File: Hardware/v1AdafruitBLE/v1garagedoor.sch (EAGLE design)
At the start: 28 parts, among them IC1 78V, Q1 2N3904, U1 ATMEGA328P_PDIP, X1 16mhz

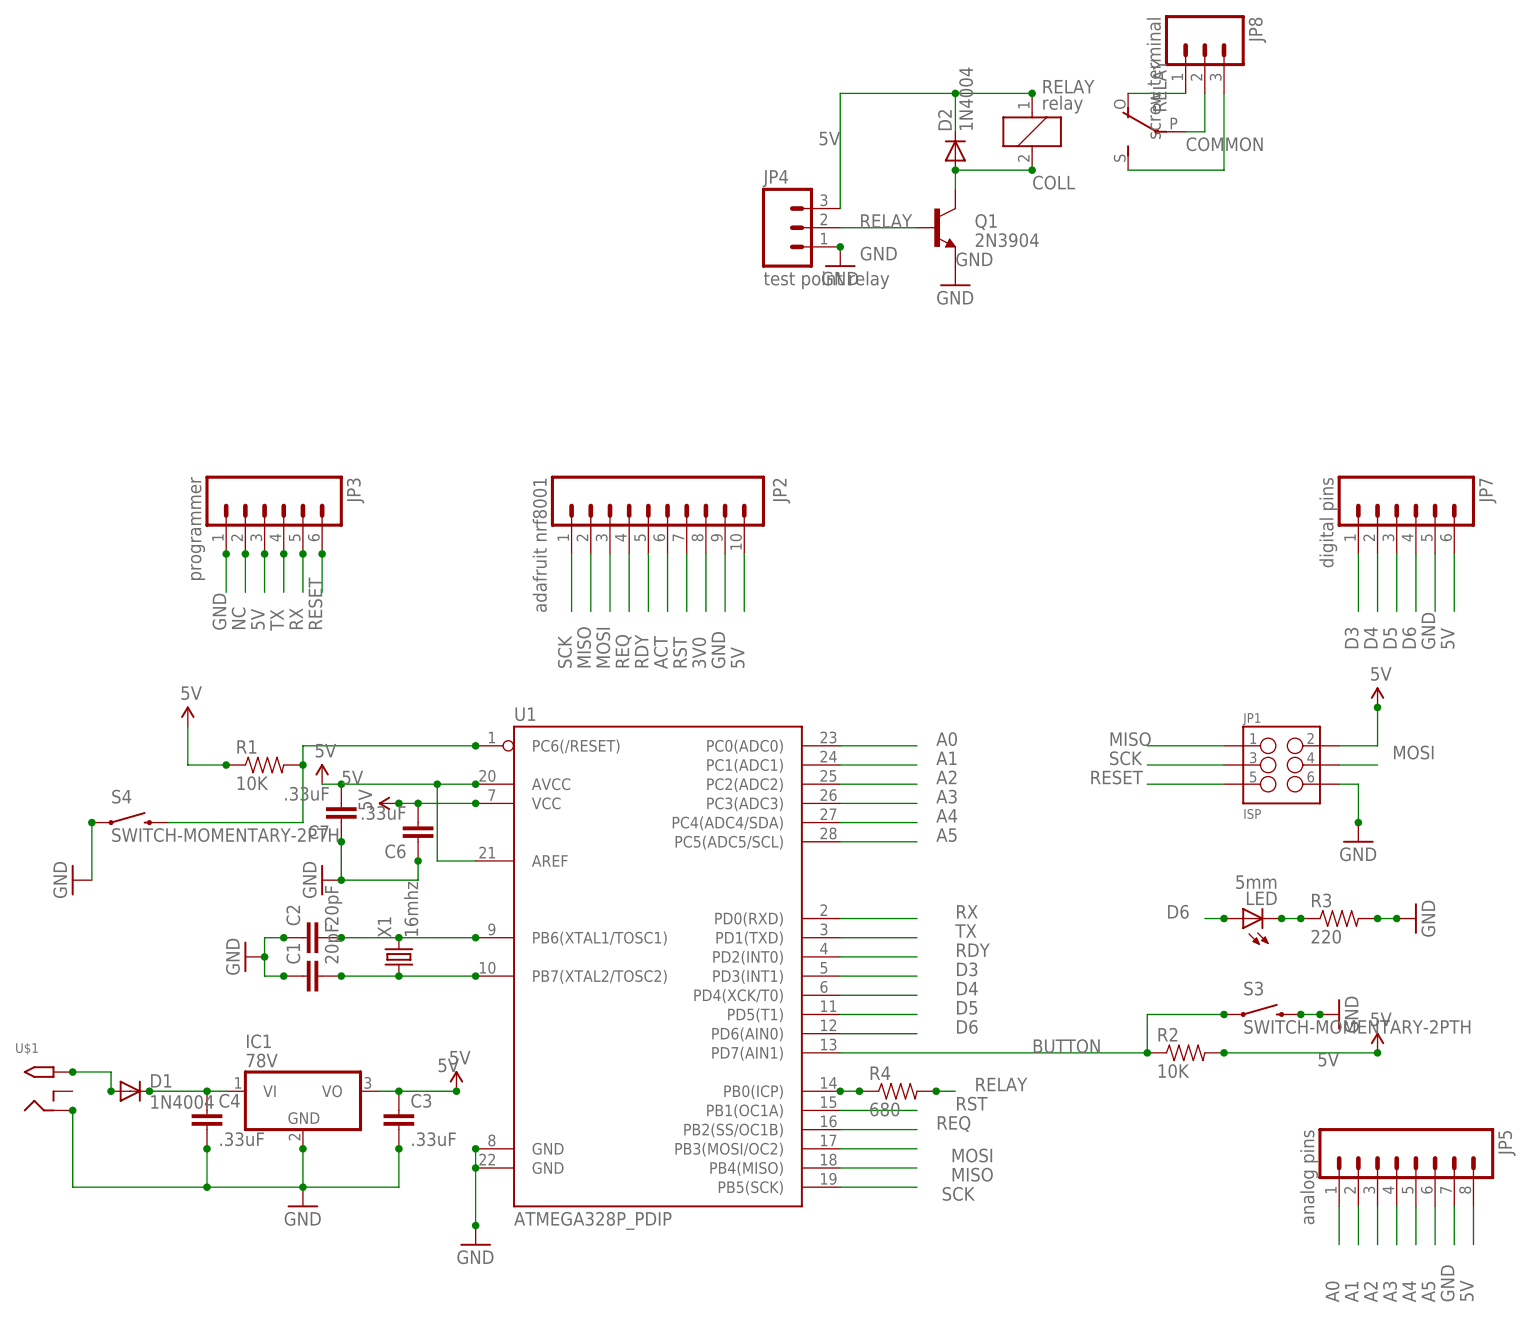
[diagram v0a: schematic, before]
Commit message: just updating the repo
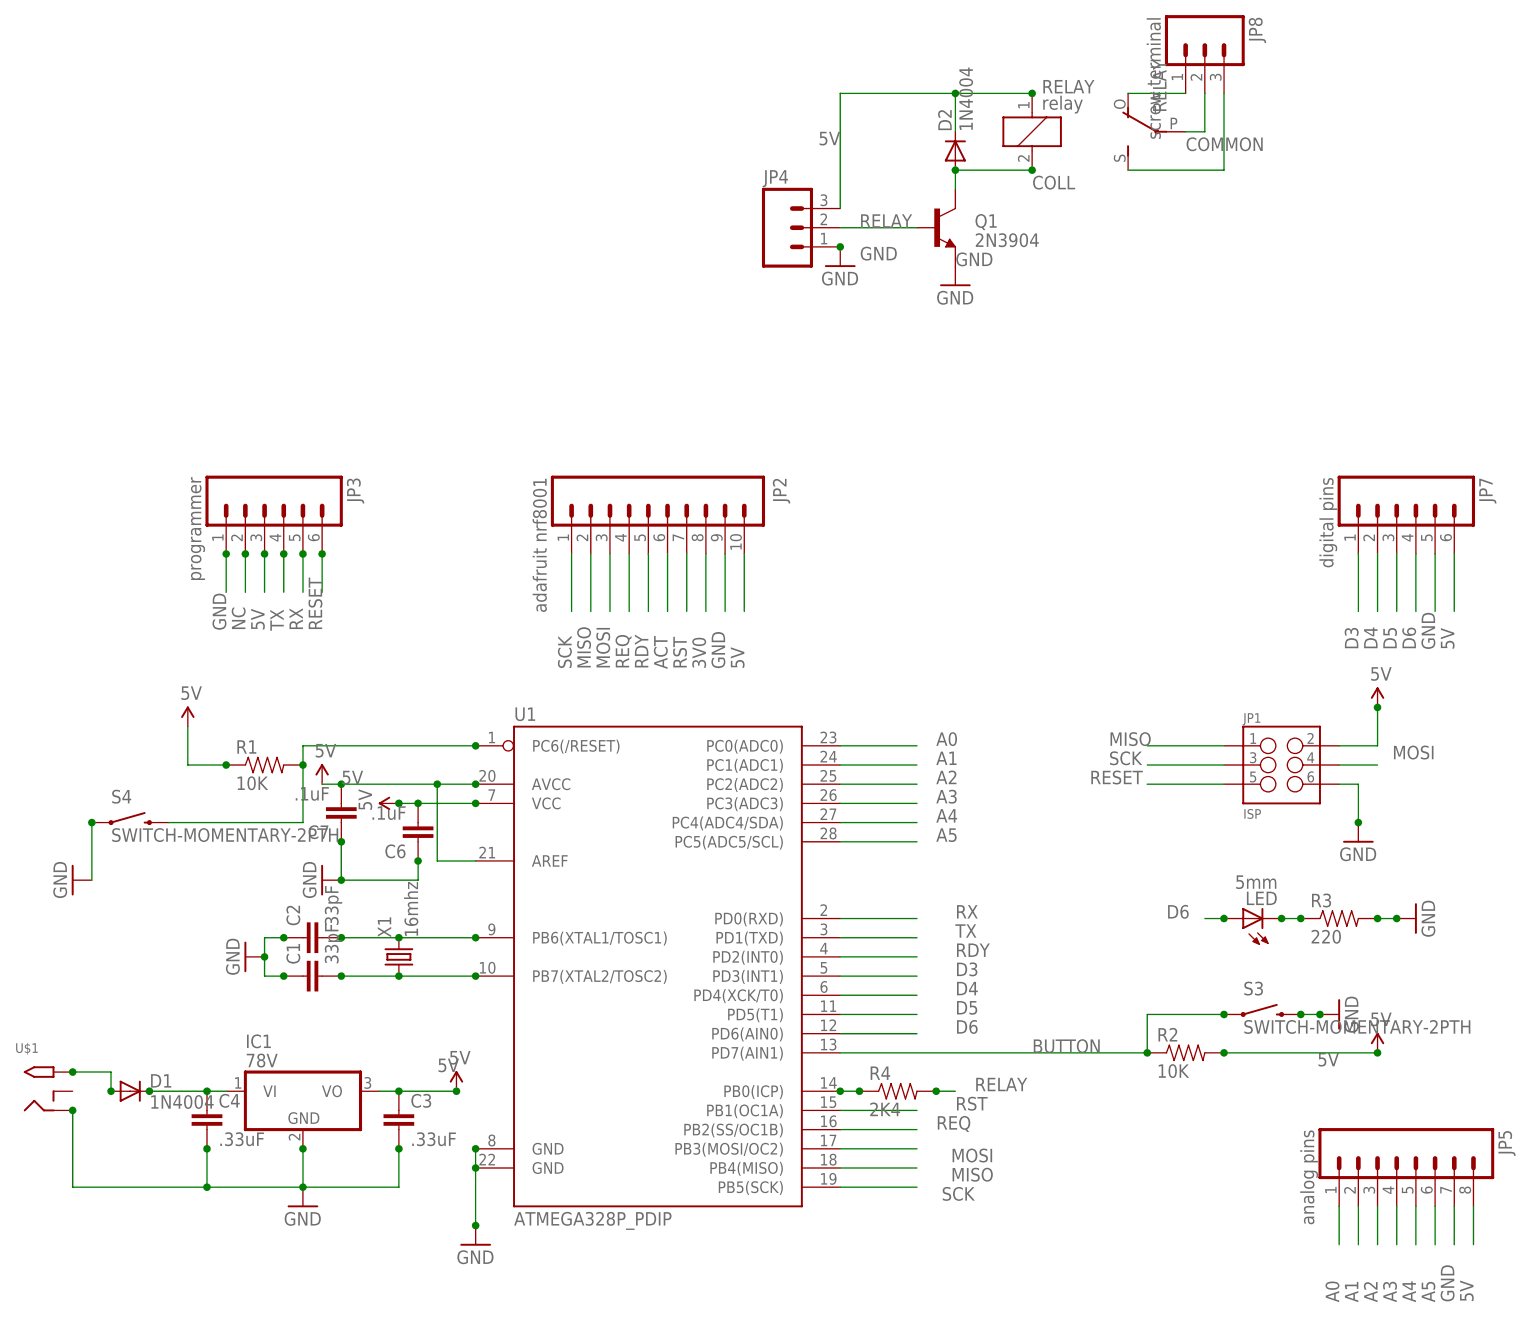
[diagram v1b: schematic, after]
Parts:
- C1, C2: value 20pF -> 33pF
- C6, C7: value .33uF -> .1uF
- JP4: value test point relay -> (none)
- R4: value 680 -> 2K4
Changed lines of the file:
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@@
 <attribute name="MOUSER" value="520-160-20-46X"/>
 </part>
-<part name="C1" library="SparkFun-Capacitors" deviceset="CAP" device="PTH1" value="20pF">
+<part name="C1" library="SparkFun-Capacitors" deviceset="CAP" device="PTH1" value="33pF">
 <attribute name="MOUSER" value="594-S200K25SL0N63L6R"/>
 </part>
-<part name="C2" library="SparkFun-Capacitors" deviceset="CAP" device="PTH1" value="20pF">
+<part name="C2" library="SparkFun-Capacitors" deviceset="CAP" device="PTH1" value="33pF">
 <attribute name="MOUSER" value="594-S200K25SL0N63L6R"/>
 </part>
@@
 <attribute name="MOUSER" value="810-FK18X5R1A334K"/>
 </part>
-<part name="C6" library="SparkFun-Capacitors" deviceset="CAP" device="KIT" value=".33uF">
+<part name="C6" library="SparkFun-Capacitors" deviceset="CAP" device="KIT" value=".1uF">
 <attribute name="MOUSER" value="810-FK18X5R1A334K"/>
 </part>
-<part name="C7" library="SparkFun-Capacitors" deviceset="CAP" device="KIT" value=".33uF">
+<part name="C7" library="SparkFun-Capacitors" deviceset="CAP" device="KIT" value=".1uF">
 <attribute name="MOUSER" value="810-FK18X5R1A334K"/>
 </part>
@@
 <part name="SUPPLY6" library="SparkFun-Aesthetics" deviceset="5V" device=""/>
 <part name="SUPPLY7" library="SparkFun-Aesthetics" deviceset="5V" device=""/>
-<part name="JP4" library="SparkFun-Connectors" deviceset="M03" device="LOCK" value="test point relay"/>
+<part name="JP4" library="SparkFun-Connectors" deviceset="M03" device="LOCK"/>
 <part name="S3" library="SparkFun-Electromechanical" deviceset="SWITCH-MOMENTARY-2" device="PTH">
 <attribute name="MOUSER" value="693-1301.9301"/>
@@
 <attribute name="MOUSER" value="655-ORWH-SH105D1F000"/>
 </part>
-<part name="R4" library="SparkFun-Resistors" deviceset="RESISTOR" device="AXIAL-0.3" value="680">
+<part name="R4" library="SparkFun-Resistors" deviceset="RESISTOR" device="AXIAL-0.3" value="2K4">
 <attribute name="MOUSER" value="603-CFR-25JR-52-680R"/>
 </part>
